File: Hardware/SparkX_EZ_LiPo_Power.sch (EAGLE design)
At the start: 40 parts, among them J3 AVR_SPI_PROG_3X2TESTPOINTS, Q1 3.1A/30V/105mΩ, U1 ATTINY43_QFN20, U2 MCP73831, U3 3.3V, U4 MAX17048

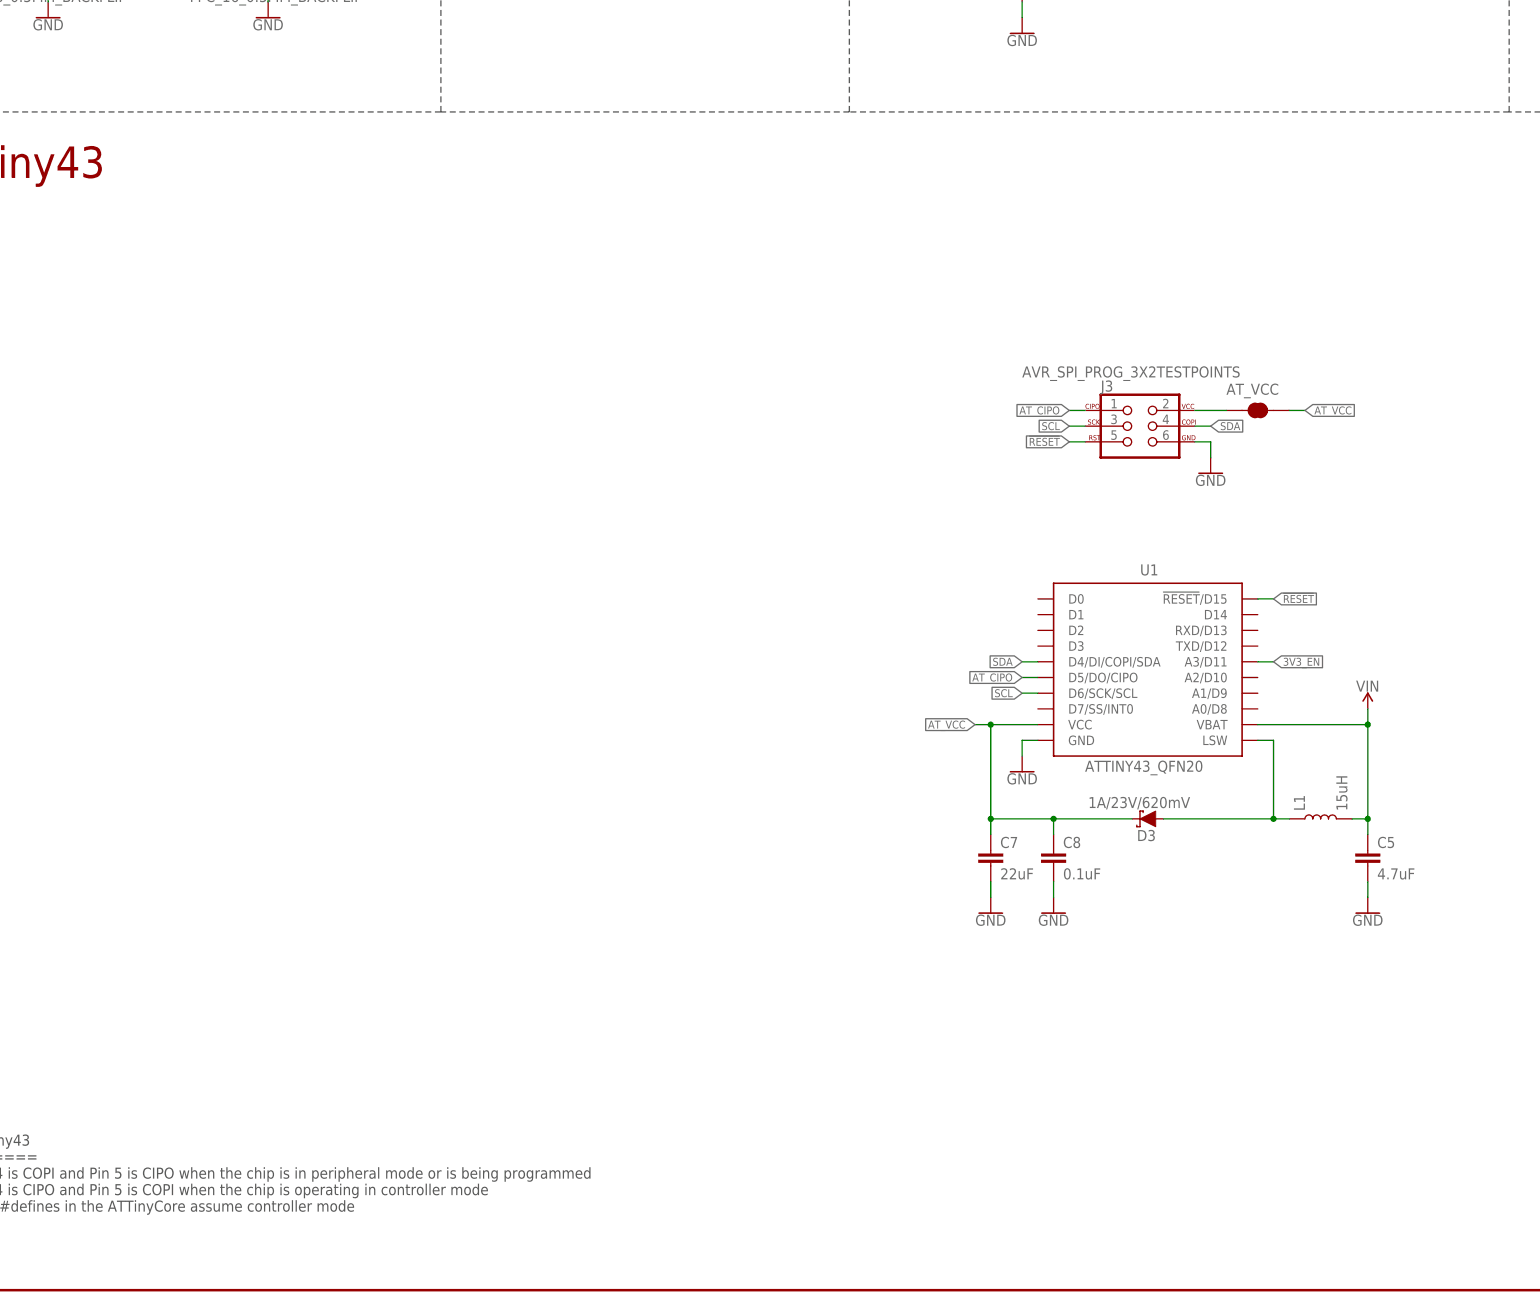
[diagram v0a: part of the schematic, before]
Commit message: Freshly routed
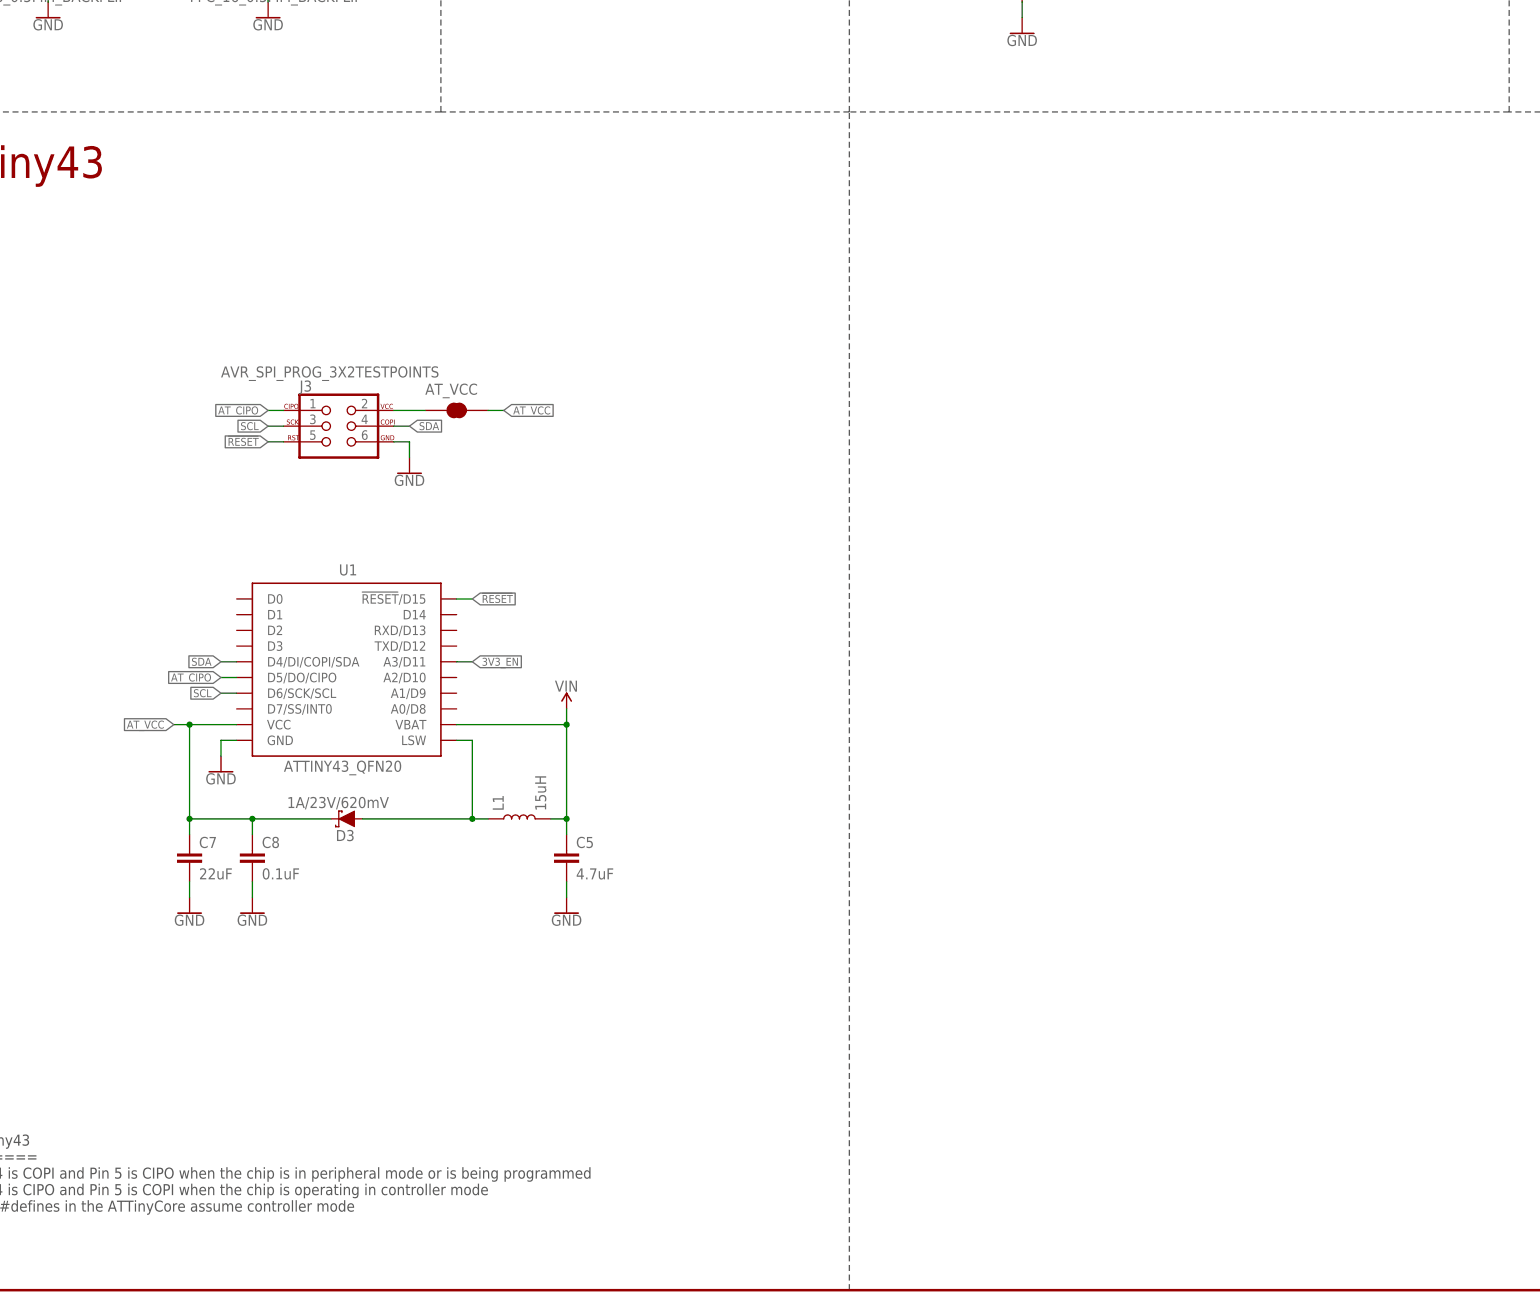
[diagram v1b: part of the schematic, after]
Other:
- moved on the sheet: AT_VCC, C5, C7, C8, D3, J3, L1, U1
